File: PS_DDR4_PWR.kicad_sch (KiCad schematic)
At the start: 2 parts, among them U12 K4A8G165WC-BCTD

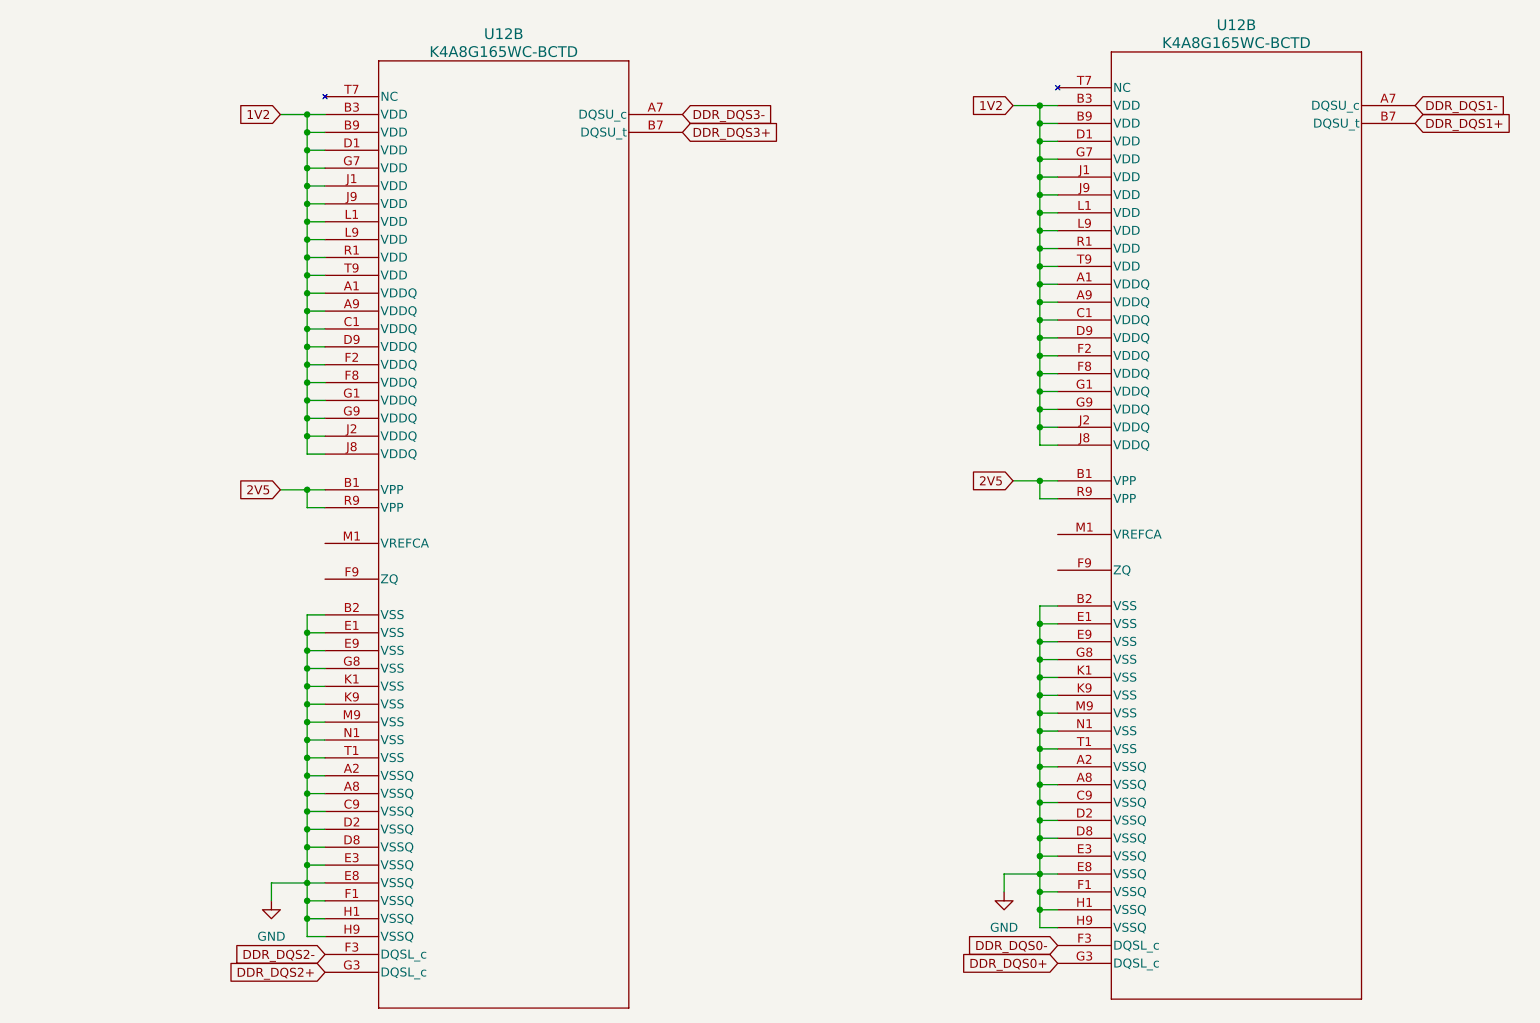
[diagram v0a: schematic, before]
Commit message: DDR4 finish
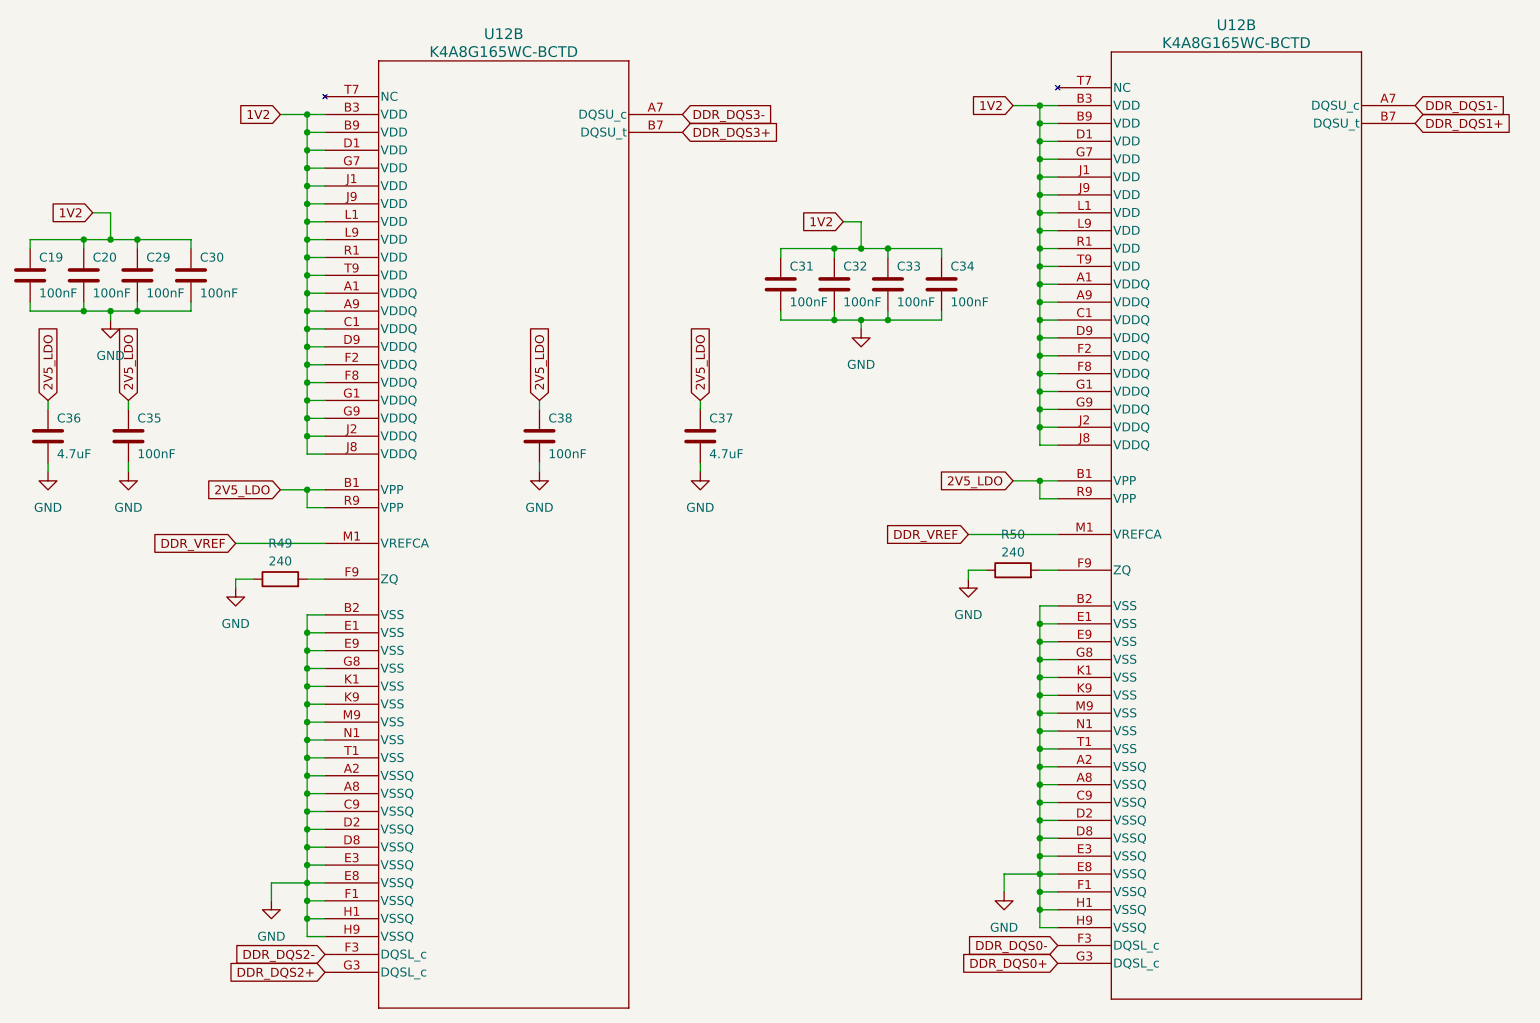
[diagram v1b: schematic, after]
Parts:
- added C19, C20, C29, C30, C31, C32, C33, C34, C35, C38: 100nF, Capacitor_SMD:C_0402_1005Metric, symbol Device:C
- added C36, C37: 4.7uF, Capacitor_SMD:C_0603_1608Metric, symbol Device:C
- added R49, R50: 240, Resistor_SMD:R_0402_1005Metric, symbol Device:R
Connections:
- net 1V2: now also C19.1, C20.1, C29.1, C30.1, C31.1, C32.1, C33.1, C34.1
- net GND: now also C19.2, C20.2, C29.2, C30.2, C31.2, C32.2, C33.2, C34.2, C35.2, C36.2, C37.2, C38.2, R49.1, R50.1
- net at U12.F9 (ZQ): now also R50.2
- net DDR_VREF: now reaches U12.M1 (VREFCA)
- net DDR_VREF: now also U12.M1 (VREFCA)
- net at U12.F9 (ZQ): now also R49.2
- net 2V5 renamed 2V5_LDO
- net 2V5_LDO: now also C35.1, C36.1, C37.1, C38.1
